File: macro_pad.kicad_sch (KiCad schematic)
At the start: 10 parts, among them SW1 SW_Push, SW2 SW_Push, SW3 SW_Push, SW4 SW_Push, SW5 SW_Push, SW6 SW_Push, SW7 SW_Push, SW8 SW_Push, SW9 SW_Push, U1 MOUDLE-SEEEDUINO-XIAO

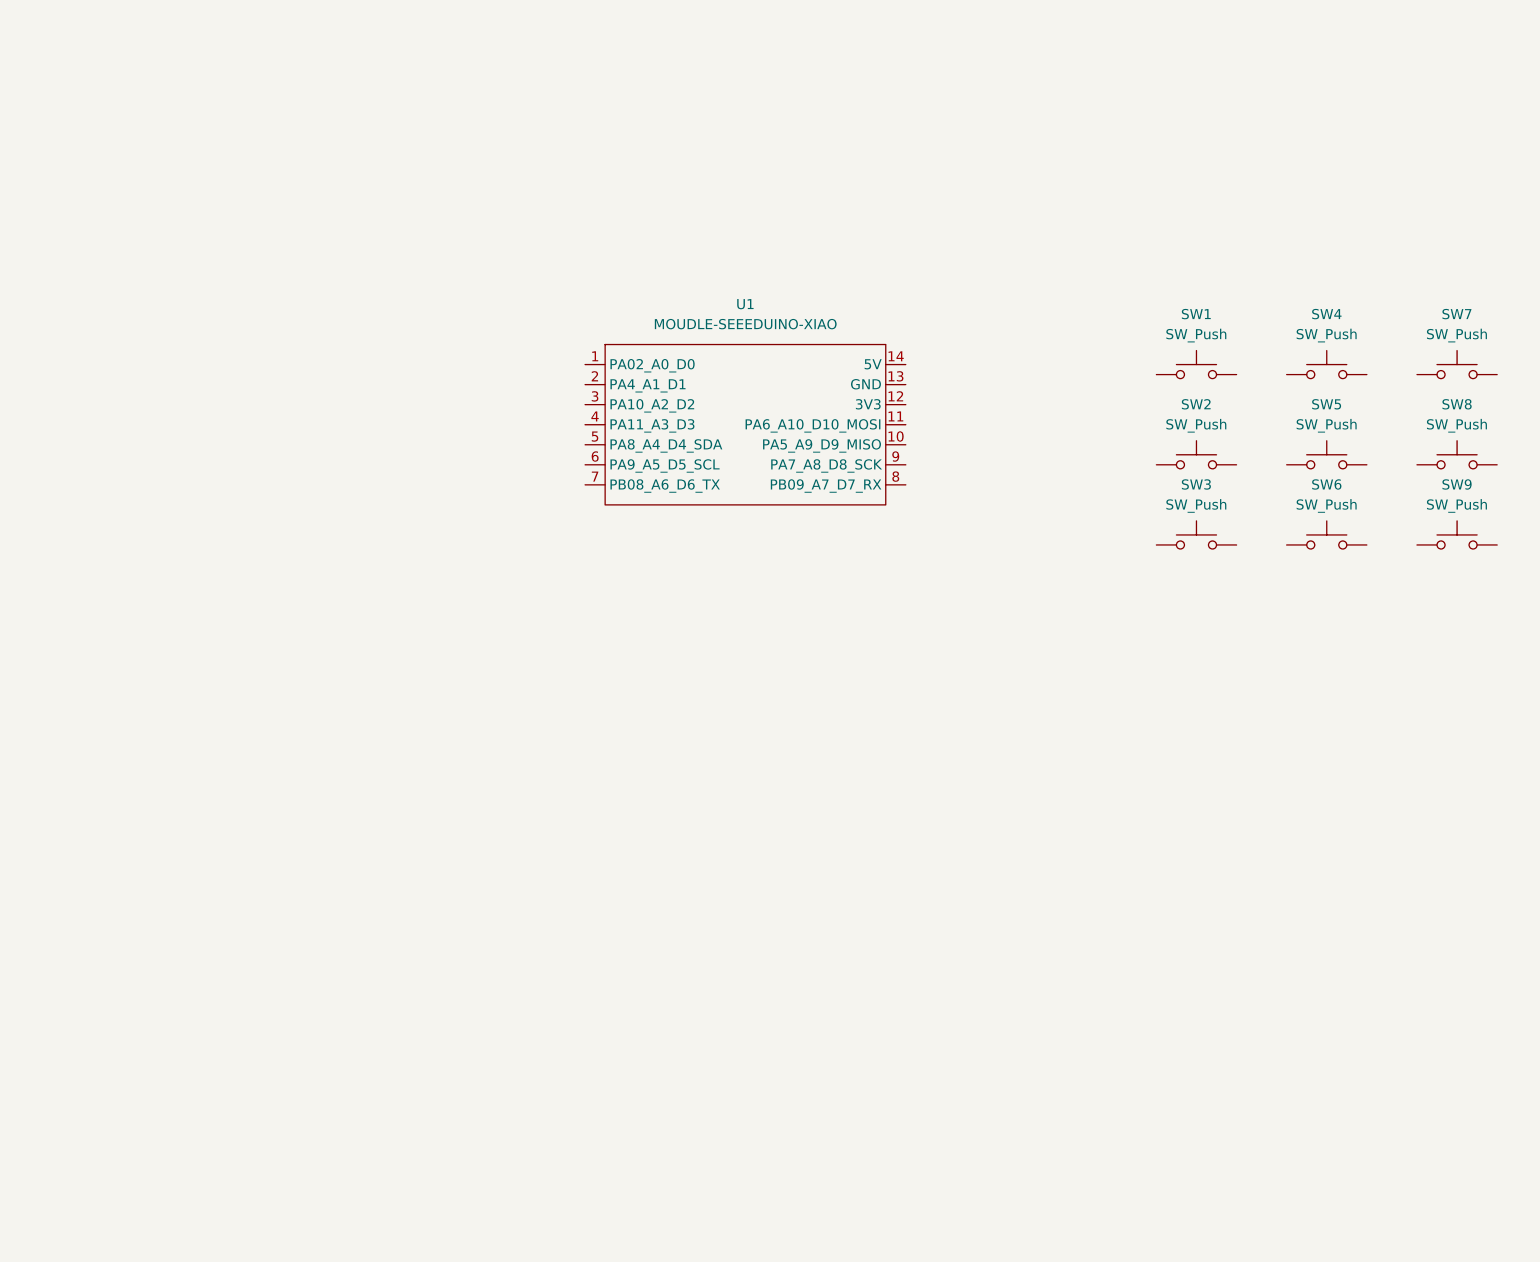
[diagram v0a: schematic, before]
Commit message: Improved design
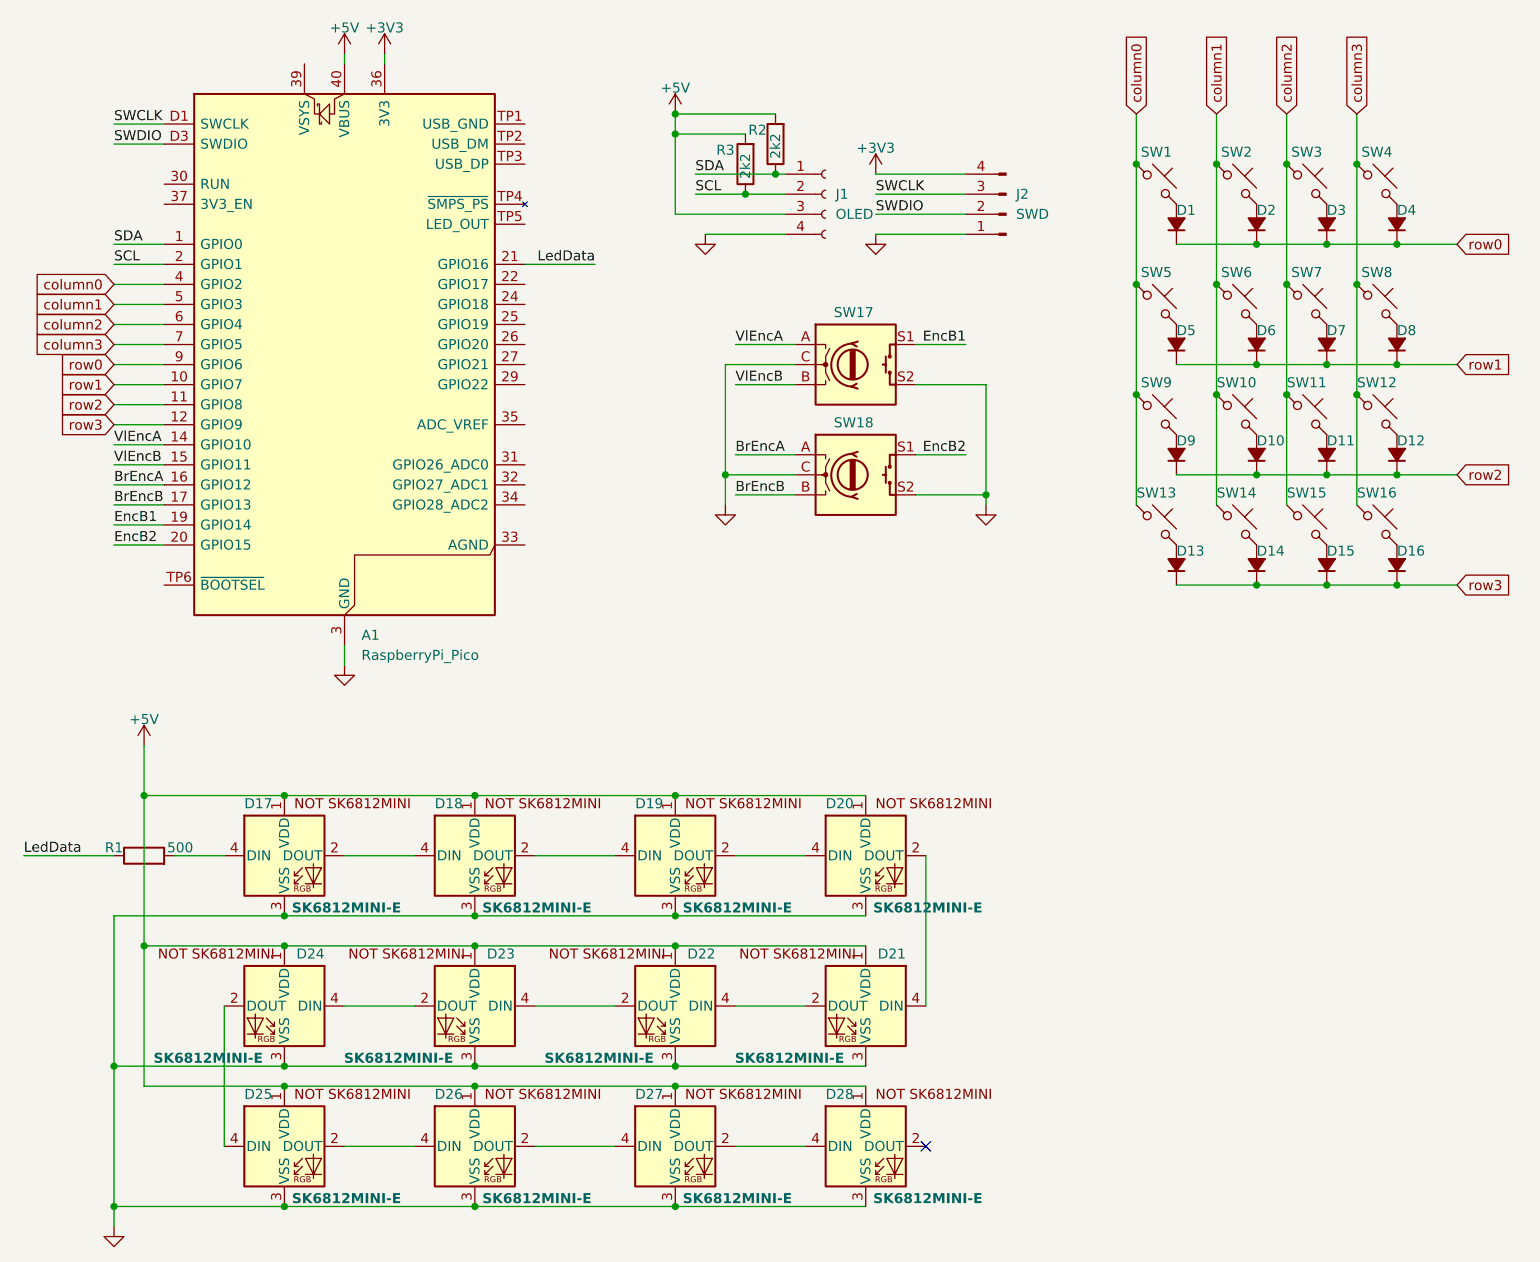
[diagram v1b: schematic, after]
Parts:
- removed SW1, SW2, SW3, SW4, SW5, SW6, SW7, SW8, SW9: SW_Push, symbol Switch:SW_Push
- removed U1: MOUDLE-SEEEDUINO-XIAO, XIAO_RP2040:XIAO-Generic-Hybrid-14P-2.54-21X17.8MM, symbol XIAO_RP2040:MOUDLE-SEEEDUINO-XIAO
- added A1: RaspberryPi_Pico, Module:RaspberryPi_Pico_SMD, symbol MCU_Module:RaspberryPi_Pico_Extensive
- added D1, D10, D11, D12, D13, D14, D15, D16, D2, D3, D4, D5, D6, D7, D8, D9: D_Small_Filled, Diode_THT:D_DO-35_SOD27_P7.62mm_Horizontal, symbol Device:D_Small_Filled
- added D17, D18, D19, D20, D21, D22, D23, D24, D25, D26, D27, D28: SK6812MINI-E, SK6812MINI-E:SK6812MINI-E_fixed, symbol SK6812MINI-E:SK6812MINI-E
- added J1: OLED, Connector_PinSocket_2.54mm:PinSocket_1x04_P2.54mm_Vertical, symbol Connector:Conn_01x04_Socket
- added J2: SWD, Connector_PinHeader_2.54mm:PinHeader_1x04_P2.54mm_Vertical, symbol Connector:Conn_01x04_Pin
- added R1: 500, Resistor_THT:R_Axial_DIN0204_L3.6mm_D1.6mm_P7.62mm_Horizontal, symbol Device:R
- added R2, R3: 2k2, Resistor_THT:R_Axial_DIN0204_L3.6mm_D1.6mm_P7.62mm_Horizontal, symbol Device:R
- added SW1, SW10, SW11, SW12, SW13, SW14, SW15, SW16, SW2, SW3, SW4, SW5, SW6, SW7, SW8, SW9: SW_Push_45deg, Button_Switch_Keyboard:SW_Cherry_MX_1.00u_PCB, symbol Switch:SW_Push_45deg
- added SW17, SW18: RotaryEncoder_Switch, RotaryEncoder_Alps_EC11E-Switch_Vertical_H20mm:RotaryEncoder_Alps_EC11E-Switch_Vertical_H20mm, symbol Device:RotaryEncoder_Switch
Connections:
- new net: D14.2 (A), SW14.2
- new net: D1.2 (A), SW1.2
- new net: D5.2 (A), SW5.2
- new net: D11.2 (A), SW11.2
- new net: D16.2 (A), SW16.2
- new net: D15.2 (A), SW15.2
- new net: D18.2 (DOUT), D19.4 (DIN)
- new net: D17.2 (DOUT), D18.4 (DIN)
- new net: D6.2 (A), SW6.2
- new net: D12.2 (A), SW12.2
- new net: D2.2 (A), SW2.2
- new net: D3.2 (A), SW3.2
- new net: D4.2 (A), SW4.2
- new net: D9.2 (A), SW9.2
- new net: D7.2 (A), SW7.2
- new net: D19.2 (DOUT), D20.4 (DIN)
- new net: D8.2 (A), SW8.2
- new net: D27.2 (DOUT), D28.4 (DIN)
- new net: D26.2 (DOUT), D27.4 (DIN)
- new net: D25.2 (DOUT), D26.4 (DIN)
- new net: D21.2 (DOUT), D22.4 (DIN)
- new net: D20.2 (DOUT), D21.4 (DIN)
- new net: D13.2 (A), SW13.2
- new net: D10.2 (A), SW10.2
- new net: D22.2 (DOUT), D23.4 (DIN)
- new net: D24.2 (DOUT), D25.4 (DIN)
- new net: D23.2 (DOUT), D24.4 (DIN)
- new net: D17.4 (DIN), R1.2
- new net +3V3: A1.36 (3V3), J2.4 (Pin_4)
- new net +5V: A1.40 (VBUS), D17.1 (VDD), D18.1 (VDD), D19.1 (VDD), D20.1 (VDD), D21.1 (VDD), D22.1 (VDD), D23.1 (VDD), D24.1 (VDD), D25.1 (VDD), D26.1 (VDD), D27.1 (VDD), D28.1 (VDD), J1.3 (Pin_3), R2.2, R3.2
- new net BrEncA: A1.16 (GPIO12), SW18.A
- new net BrEncB: A1.17 (GPIO13), SW18.B
- new net EncB1: A1.19 (GPIO14), SW17.S1
- new net EncB2: A1.20 (GPIO15), SW18.S1
- new net GND: A1.13 (GND), A1.18 (GND), A1.23 (GND), A1.28 (GND), A1.3 (GND), A1.38 (GND), A1.8 (GND), A1.D2 (GND), D17.3 (VSS), D18.3 (VSS), D19.3 (VSS), D20.3 (VSS), D21.3 (VSS), D22.3 (VSS), D23.3 (VSS), D24.3 (VSS), D25.3 (VSS), D26.3 (VSS), D27.3 (VSS), D28.3 (VSS), J1.4 (Pin_4), J2.1 (Pin_1), SW17.C, SW17.S2, SW18.C, SW18.S2
- new net LedData: A1.21 (GPIO16), R1.1
- new net SCL: A1.2 (GPIO1), J1.2 (Pin_2), R3.1
- new net SDA: A1.1 (GPIO0), J1.1 (Pin_1), R2.1
- new net SWCLK: A1.D1 (SWCLK), J2.3 (Pin_3)
- new net SWDIO: A1.D3 (SWDIO), J2.2 (Pin_2)
- new net VlEncA: A1.14 (GPIO10), SW17.A
- new net VlEncB: A1.15 (GPIO11), SW17.B
- new net column0: A1.4 (GPIO2), SW1.1, SW13.1, SW5.1, SW9.1
- new net column1: A1.5 (GPIO3), SW10.1, SW14.1, SW2.1, SW6.1
- new net column2: A1.6 (GPIO4), SW11.1, SW15.1, SW3.1, SW7.1
- new net column3: A1.7 (GPIO5), SW12.1, SW16.1, SW4.1, SW8.1
- new net row0: A1.9 (GPIO6), D1.1 (K), D2.1 (K), D3.1 (K), D4.1 (K)
- new net row1: A1.10 (GPIO7), D5.1 (K), D6.1 (K), D7.1 (K), D8.1 (K)
- new net row2: A1.11 (GPIO8), D10.1 (K), D11.1 (K), D12.1 (K), D9.1 (K)
- new net row3: A1.12 (GPIO9), D13.1 (K), D14.1 (K), D15.1 (K), D16.1 (K)
- no-connect marks 0 -> 1
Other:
- company: (none) -> Hackclub
- title: (none) -> Macropad
